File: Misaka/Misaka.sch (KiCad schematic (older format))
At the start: 4 parts, among them J1 Conn_Coaxial_Power, SW1 SW_DIP_x03, U2 ATmega2560-16AU

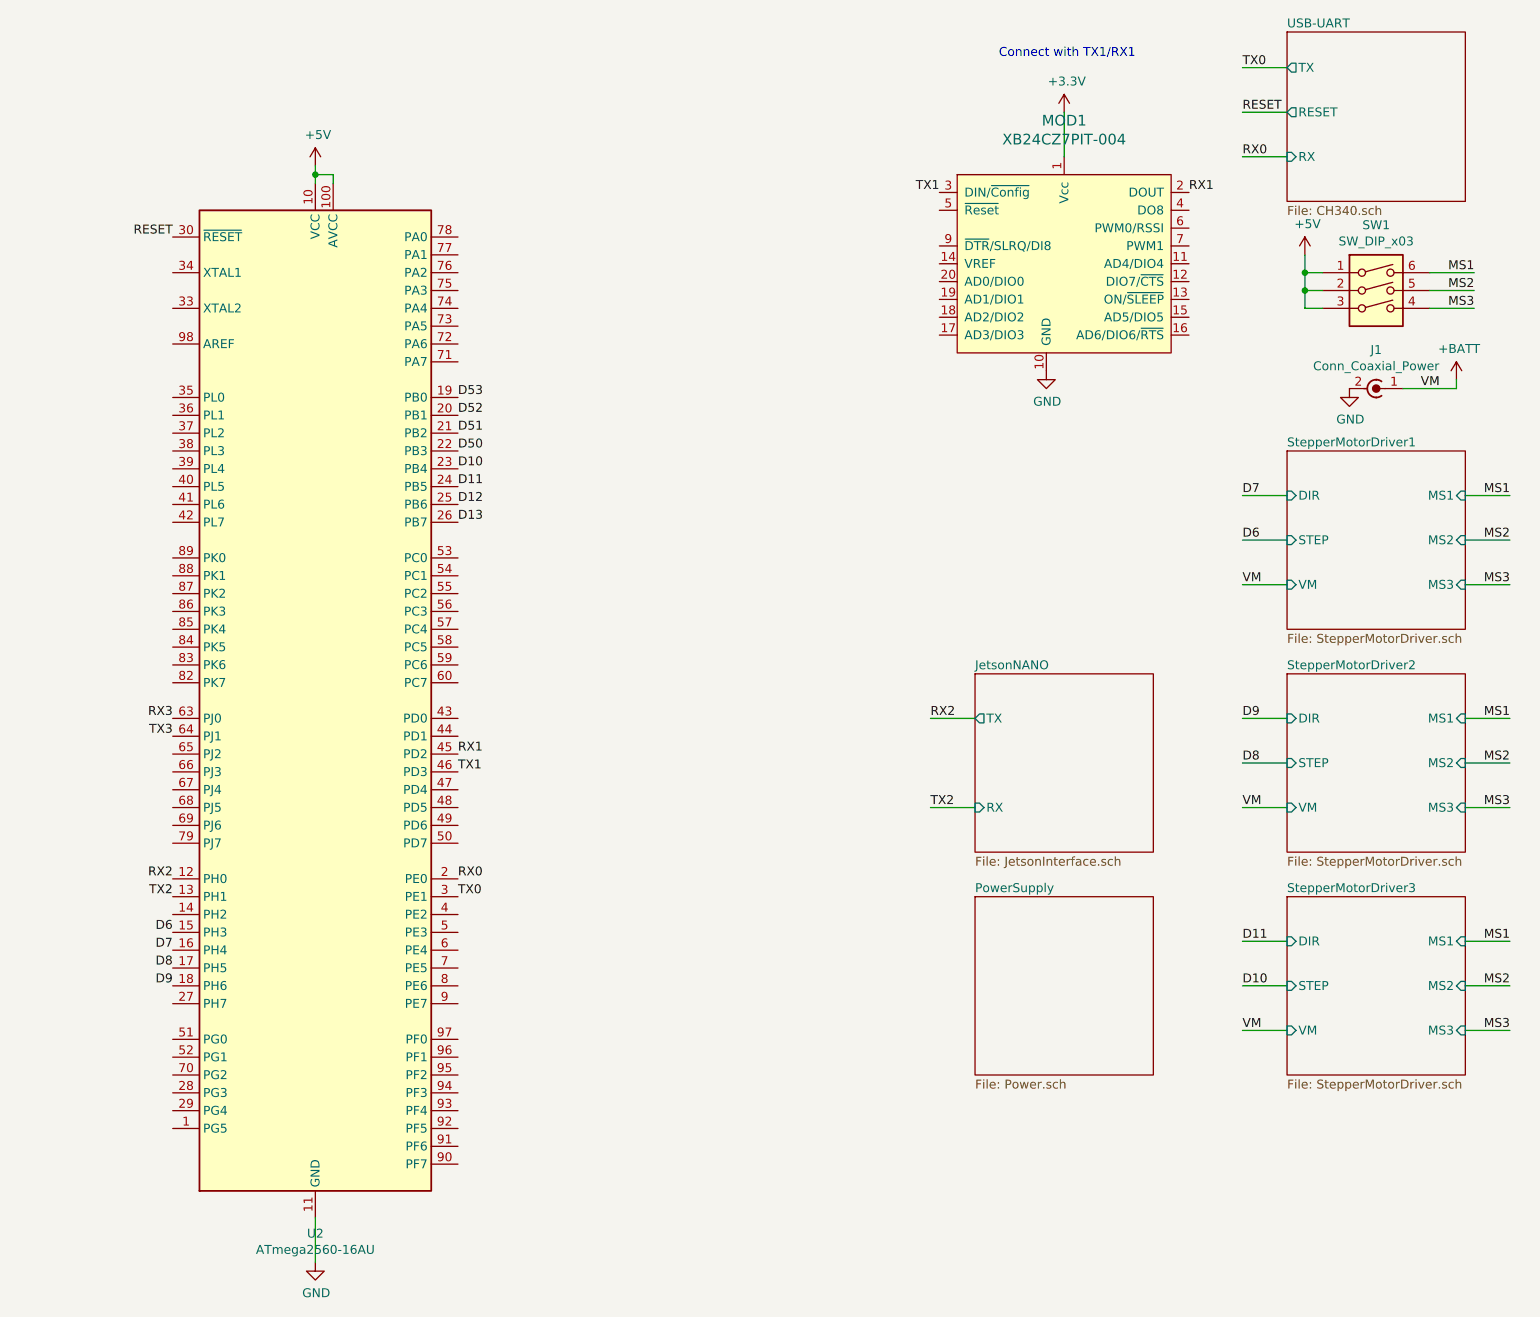
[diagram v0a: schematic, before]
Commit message: V1
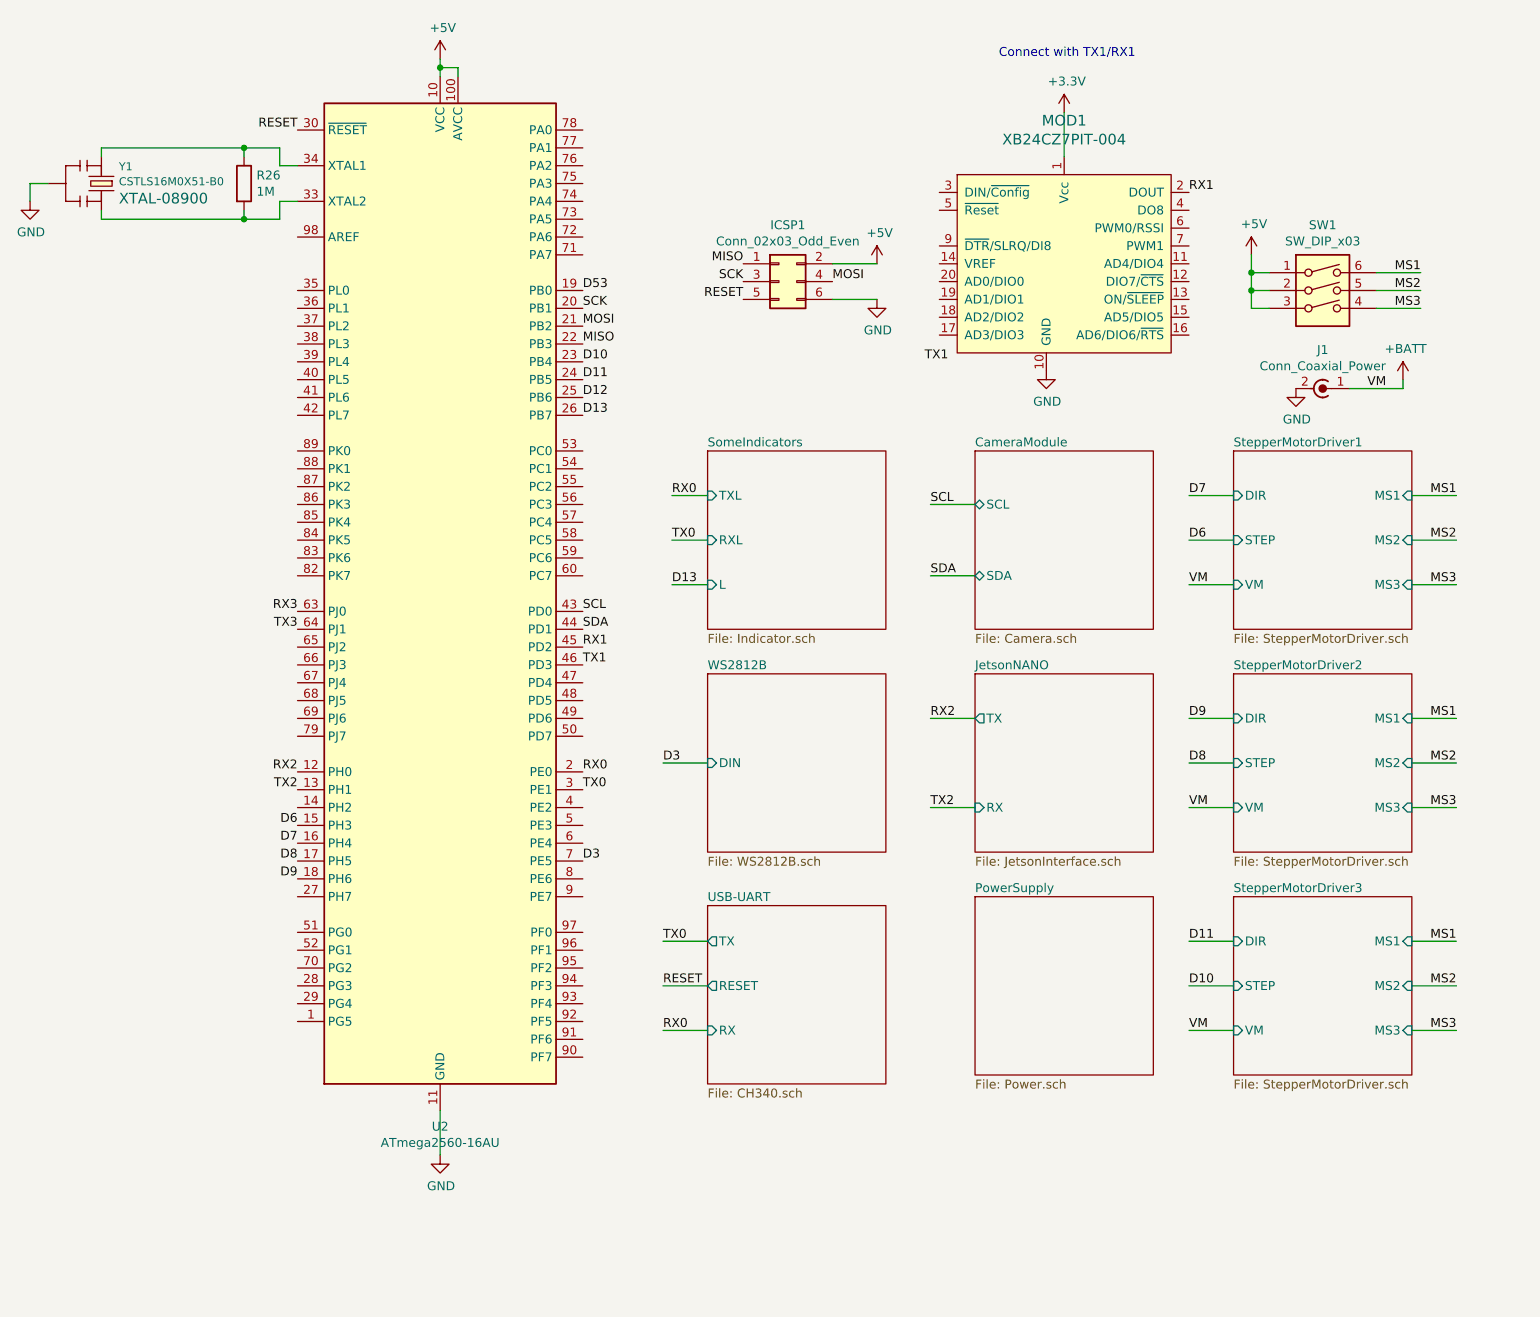
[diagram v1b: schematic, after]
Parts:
- added ICSP1: Conn_02x03_Odd_Even, Connector_PinHeader_2.54mm:PinHeader_2x03_P2.54mm_Vertical, symbol Connector_Generic:Conn_02x03_Odd_Even
- added R26: 1M, Resistor_SMD:R_0603_1608Metric_Pad1.05x0.95mm_HandSolder, symbol Device:R
- added Y1: CSTLS16M0X51-B0, Crystal:Resonator_muRata_CSTLSxxxX-3Pin_W5.5mm_H3.0mm, symbol SparkFun-Clocks:RESONATOR-16MHZSMD_3.2X1.3
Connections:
- net +5V: now also ICSP1.2 (Pin_2)
- net GND: now also ICSP1.6 (Pin_6), Y1.2
- net RESET: now also ICSP1.5 (Pin_5)
- net TX1: no longer MOD1.3 (DIN/~Config)
- net at U2.33 (XTAL2): now also R26.2, Y1.3
- net at U2.34 (XTAL1): now also R26.1, Y1.1
- net SCL: now reaches U2.43 (PD0)
- net SDA: now reaches U2.44 (PD1)
- net D3: now reaches U2.7 (PE5)
- net D50 renamed MISO
- net MISO: now also ICSP1.1 (Pin_1)
- net D51 renamed MOSI
- net MOSI: now also ICSP1.4 (Pin_4)
- net D52 renamed SCK
- net SCK: now also ICSP1.3 (Pin_3)
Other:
- moved on the sheet: J1, SW1, U2
